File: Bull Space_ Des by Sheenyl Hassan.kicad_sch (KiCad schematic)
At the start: 24 parts, among them IC1 TEENSY_4.0, IC2 XB24CZ7PIT-004, J1 Screw_Terminal_01x06, Q4 2N7002, U1 VXO7803-1000, U2 Flight-Computer_Adafruit_GPS_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, U3 ADXL343, U4 BMP280, U6 Memory_Flash_W25Q32JVSS

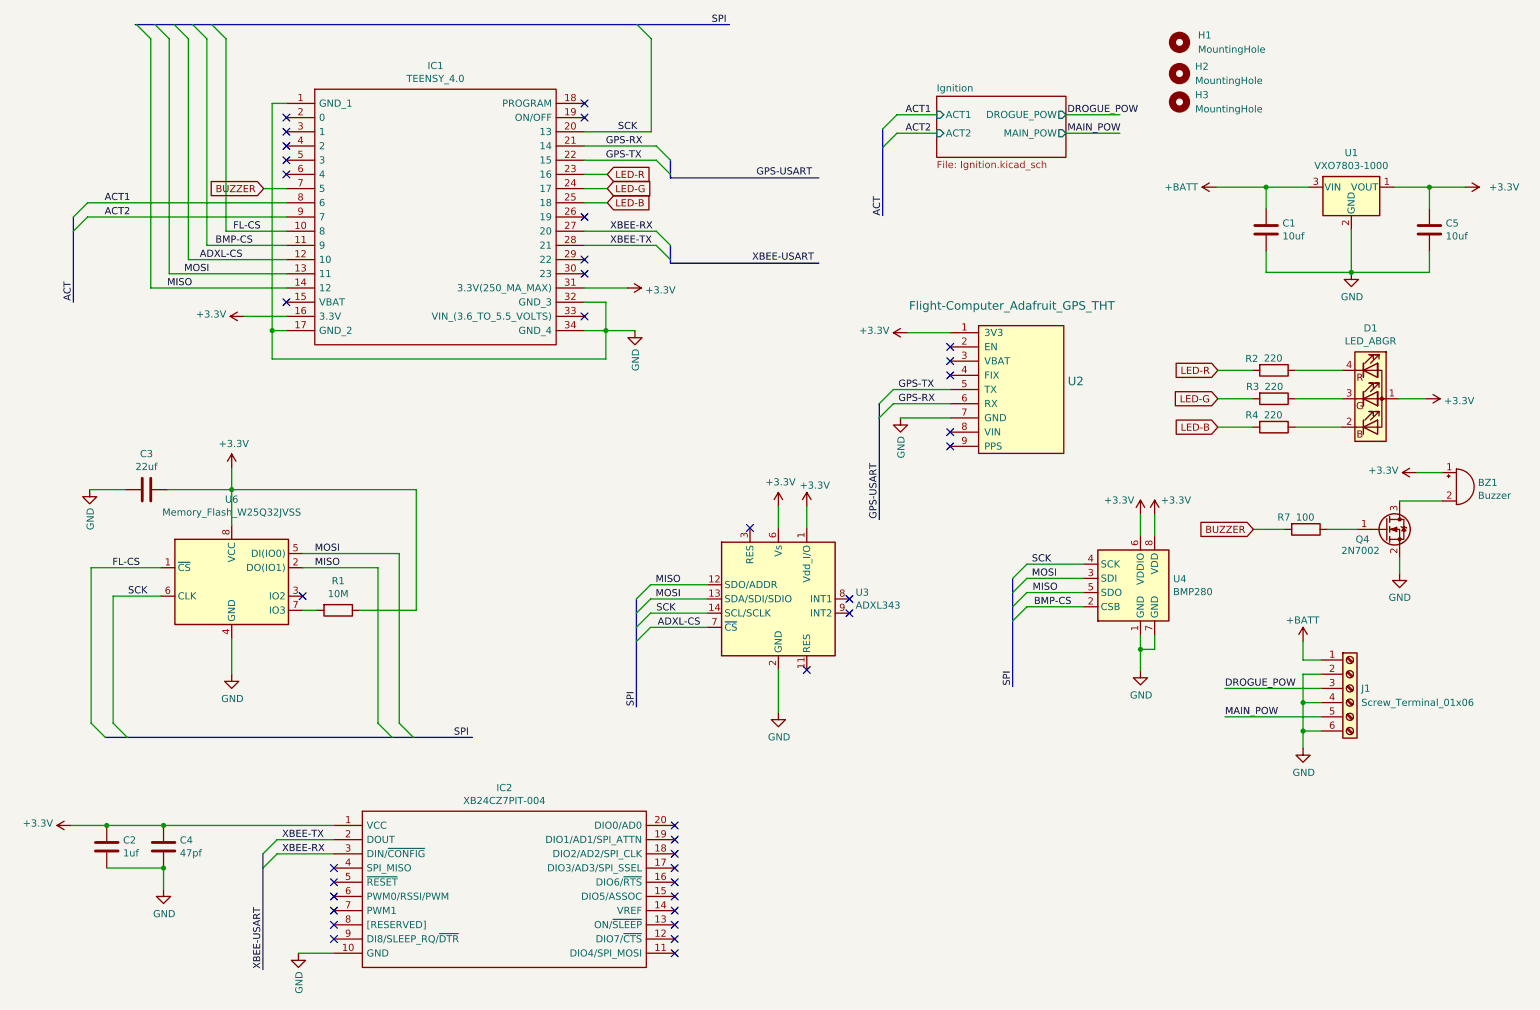
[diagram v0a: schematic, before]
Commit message: Fix schematic grid
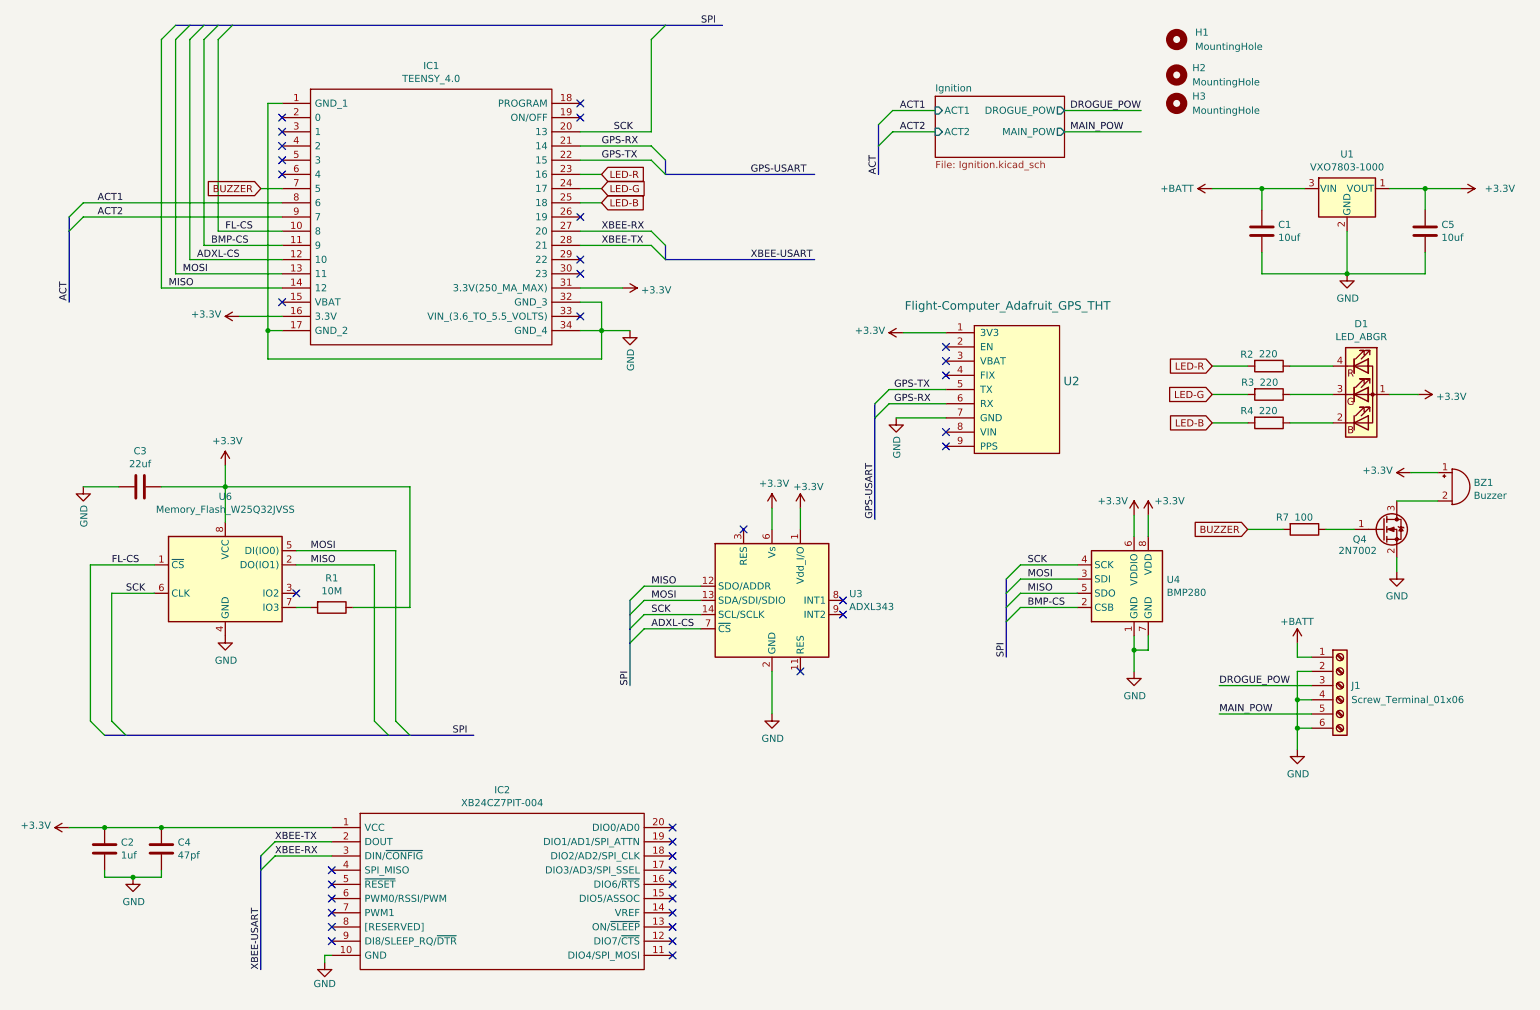
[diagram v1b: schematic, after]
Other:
- moved on the sheet: BZ1, C1, C2, C3, C4, C5, D1, H1, H2, H3, IC1, IC2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
